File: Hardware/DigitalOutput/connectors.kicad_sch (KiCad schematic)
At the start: 3 parts, among them J1 DIGITAL OUTPUT, J3 NUCLEO LEFT, J4 NUCLEO RIGHT

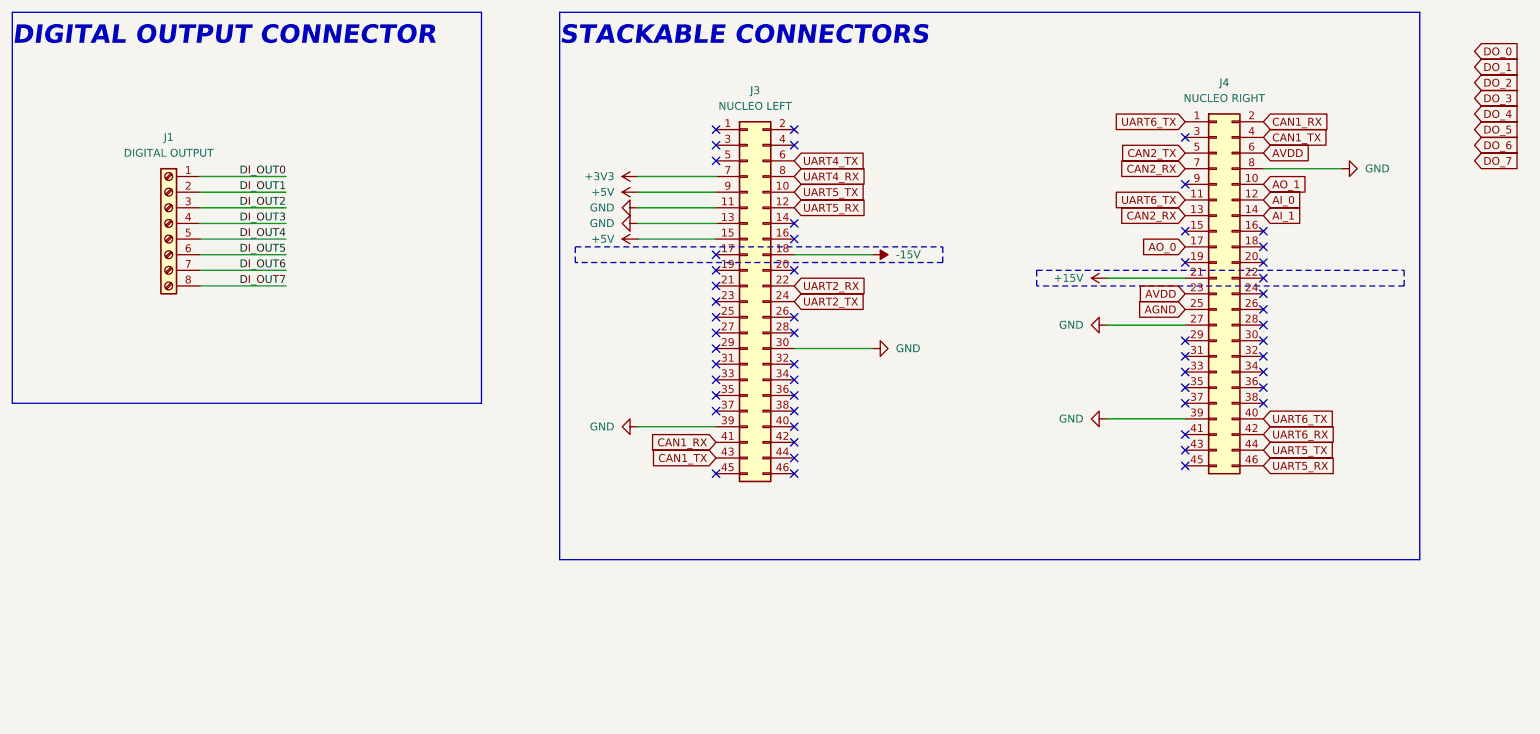
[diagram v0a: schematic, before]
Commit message: digital output & power finished
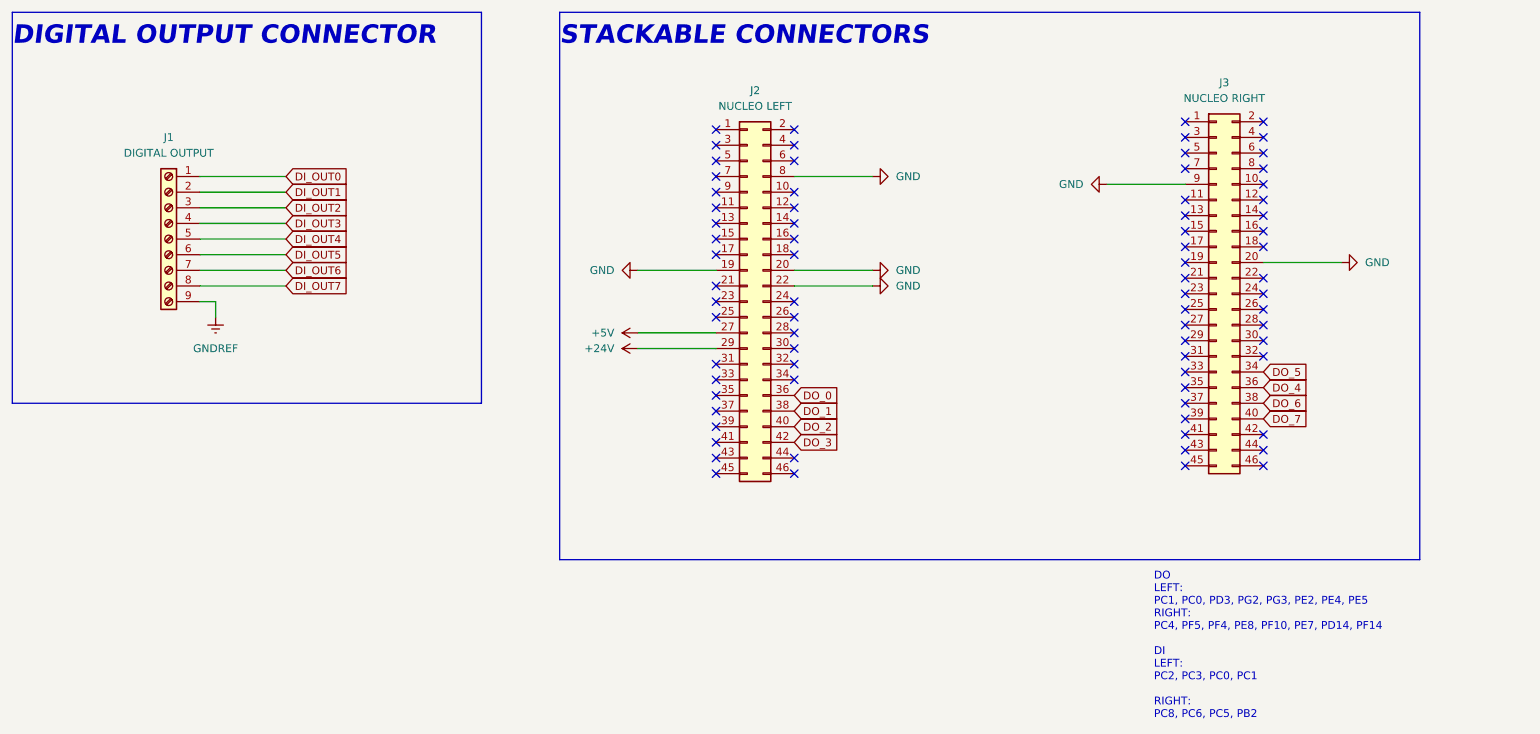
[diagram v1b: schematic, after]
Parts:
- removed J1: DIGITAL OUTPUT, PLC_STM:1725711, symbol Connector:Screw_Terminal_01x08
- added J1: DIGITAL OUTPUT, PLC_STM:1725724, symbol Connector:Screw_Terminal_01x09
- renumbered J3 to J2, J4 to J3
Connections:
- net UART2_RX is gone; now on net GND: J2.22 (Pin_22)
- net UART4_RX is gone; now on net GND: J2.8 (Pin_8)
- net +5V: now also J2.27 (Pin_27); no longer J2.15 (Pin_15), J2.9 (Pin_9)
- net DI_OUT0: now also J1.1 (Pin_1)
- net DI_OUT1: now also J1.2 (Pin_2)
- net DI_OUT2: now also J1.3 (Pin_3)
- net DI_OUT3: now also J1.4 (Pin_4)
- net DI_OUT4: now also J1.5 (Pin_5)
- net DI_OUT5: now also J1.6 (Pin_6)
- net DI_OUT6: now also J1.7 (Pin_7)
- net DI_OUT7: now also J1.8 (Pin_8)
- net DO_0: now also J2.36 (Pin_36)
- net DO_1: now also J2.38 (Pin_38)
- net DO_2: now also J2.40 (Pin_40)
- net DO_3: now also J2.42 (Pin_42)
- net DO_4: now also J3.36 (Pin_36)
- net DO_5: now also J3.34 (Pin_34)
- net DO_6: now also J3.38 (Pin_38)
- net DO_7: now also J3.40 (Pin_40)
- net GND: now also J2.19 (Pin_19), J2.20 (Pin_20), J3.20 (Pin_20), J3.9 (Pin_9); no longer J2.11 (Pin_11), J2.13 (Pin_13), J2.30 (Pin_30), J2.39 (Pin_39), J3.27 (Pin_27), J3.39 (Pin_39), J3.8 (Pin_8)
- net +24V: now reaches J2.29 (Pin_29)
- net +15V: no longer names the net of J3.21 (Pin_21)
- net +3V3: no longer names the net of J2.7 (Pin_7)
- net -15V: no longer names the net of J2.18 (Pin_18)
- net AGND: no longer names the net of J3.25 (Pin_25)
- net AI_0: no longer names the net of J3.12 (Pin_12)
- net AI_1: no longer names the net of J3.14 (Pin_14)
- net AO_0: no longer names the net of J3.17 (Pin_17)
- net AO_1: no longer names the net of J3.10 (Pin_10)
- net AVDD: no longer names the net of J3.23 (Pin_23)
- net AVDD: no longer J3.6 (Pin_6)
- net CAN1_RX: no longer names the net of J3.2 (Pin_2)
- net CAN1_RX: no longer J2.41 (Pin_41)
- net CAN1_TX: no longer names the net of J3.4 (Pin_4)
- net CAN1_TX: no longer J2.43 (Pin_43)
- net CAN2_RX: no longer names the net of J3.13 (Pin_13)
- net CAN2_RX: no longer J3.7 (Pin_7)
- net CAN2_TX: no longer names the net of J3.5 (Pin_5)
- net UART2_TX: no longer names the net of J2.24 (Pin_24)
- net UART4_TX: no longer names the net of J2.6 (Pin_6)
- net UART5_RX: no longer names the net of J3.46 (Pin_46)
- net UART5_RX: no longer J2.12 (Pin_12)
- net UART5_TX: no longer names the net of J3.44 (Pin_44)
- net UART5_TX: no longer J2.10 (Pin_10)
- net UART6_RX: no longer names the net of J3.42 (Pin_42)
- removed net UART6_TX: J3.1 (Pin_1), J3.11 (Pin_11), J3.40 (Pin_40)
- new net GNDREF: J1.9 (Pin_9)
- no-connect marks 54 -> 76
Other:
- note added: "DO LEFT: PC1, PC0, PD3, PG2, PG3, PE2, PE4, PE5 RIGHT: PC4, PF5, PF4, PE8, PF10, PE7, PD14, PF14 DI LEFT: PC2, PC3, PC0, PC1 RIGHT: PC8, PC6, PC5, PB2"

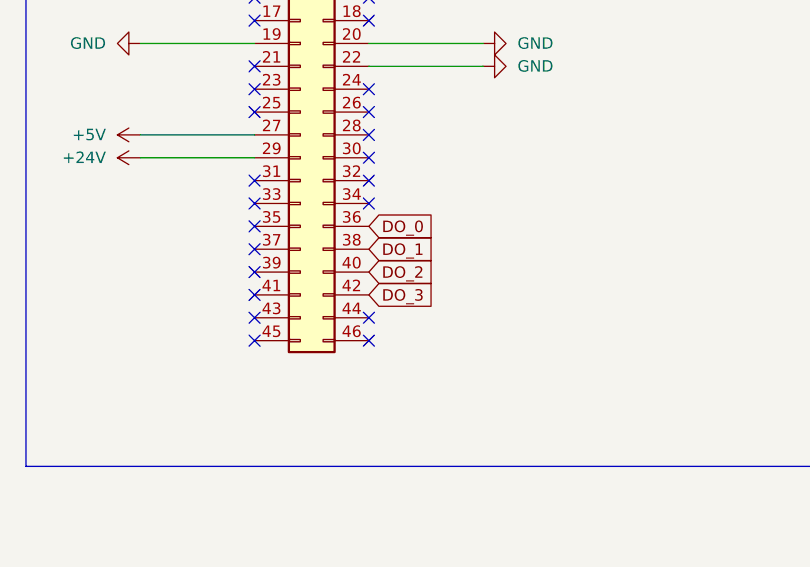
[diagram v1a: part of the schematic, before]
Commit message: small adjustments and final revision
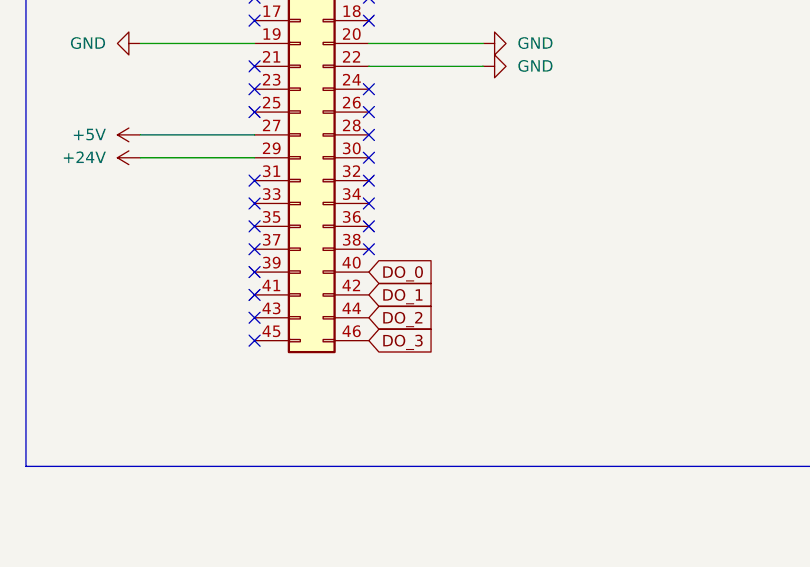
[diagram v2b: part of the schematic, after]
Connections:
- net DO_0: now also J2.40 (Pin_40); no longer J2.36 (Pin_36)
- net DO_1: now also J2.42 (Pin_42); no longer J2.38 (Pin_38)
- net DO_2: now also J2.44 (Pin_44); no longer J2.40 (Pin_40)
- net DO_3: now also J2.46 (Pin_46); no longer J2.42 (Pin_42)
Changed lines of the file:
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@@
-	)
-	(no_connect
-		(at 165.1 110.49)
 	)
 	(no_connect
@@
 	)
 	(no_connect
-		(at 165.1 113.03)
+		(at 165.1 102.87)
 	)
 	(no_connect
@@
 	)
 	(no_connect
+		(at 165.1 100.33)
+	)
+	(no_connect
 		(at 241.3 91.44)
 	)
@@
 		)
 	)
+	(global_label "DO_1"
+		(shape input)
+		(at 165.1 107.95 0)
+		(fields_autoplaced yes)
+		(effects
+			(font
+				(size 1.27 1.27)
+			)
+			(justify left)
+		)
+		(property "Intersheetrefs" "${INTERSHEET_REFS}"
+			(at 172.8628 107.95 0)
+			(effects
+				(font
+					(size 1.27 1.27)
+				)
+				(justify left)
+				(hide yes)
+			)
+		)
+	)
 	(global_label "DI_OUT1"
 		(shape input)
@@
 		)
 	)
+	(global_label "DO_5"
+		(shape input)
+		(at 241.3 96.52 0)
+		(fields_autoplaced yes)
+		(effects
+			(font
+				(size 1.27 1.27)
+			)
+			(justify left)
+		)
+		(property "Intersheetrefs" "${INTERSHEET_REFS}"
+			(at 249.0628 96.52 0)
+			(effects
+				(font
+					(size 1.27 1.27)
+				)
+				(justify left)
+				(hide yes)
+			)
+		)
+	)
 	(global_label "DO_2"
 		(shape input)
+		(at 165.1 110.49 0)
+		(fields_autoplaced yes)
+		(effects
+			(font
+				(size 1.27 1.27)
+			)
+			(justify left)
+		)
+		(property "Intersheetrefs" "${INTERSHEET_REFS}"
+			(at 172.8628 110.49 0)
+			(effects
+				(font
+					(size 1.27 1.27)
+				)
+				(justify left)
+				(hide yes)
+			)
+		)
+	)
+	(global_label "DI_OUT2"
+		(shape input)
+		(at 82.55 69.85 0)
+		(fields_autoplaced yes)
+		(effects
+			(font
+				(size 1.27 1.27)
+			)
+			(justify left)
+		)
+		(property "Intersheetrefs" "${INTERSHEET_REFS}"
+			(at 93.2157 69.85 0)
+			(effects
+				(font
+					(size 1.27 1.27)
+				)
+				(justify left)
+				(hide yes)
+			)
+		)
+	)
+	(global_label "DO_4"
+		(shape input)
+		(at 241.3 99.06 0)
+		(fields_autoplaced yes)
+		(effects
+			(font
+				(size 1.27 1.27)
+			)
+			(justify left)
+		)
+		(property "Intersheetrefs" "${INTERSHEET_REFS}"
+			(at 249.0628 99.06 0)
+			(effects
+				(font
+					(size 1.27 1.27)
+				)
+				(justify left)
+				(hide yes)
+			)
+		)
+	)
+	(global_label "DI_OUT3"
+		(shape input)
+		(at 82.55 72.39 0)
+		(fields_autoplaced yes)
+		(effects
+			(font
+				(size 1.27 1.27)
+			)
+			(justify left)
+		)
+		(property "Intersheetrefs" "${INTERSHEET_REFS}"
+			(at 93.2157 72.39 0)
+			(effects
+				(font
+					(size 1.27 1.27)
+				)
+				(justify left)
+				(hide yes)
+			)
+		)
+	)
+	(global_label "DO_7"
+		(shape input)
+		(at 241.3 104.14 0)
+		(fields_autoplaced yes)
+		(effects
+			(font
+				(size 1.27 1.27)
+			)
+			(justify left)
+		)
+		(property "Intersheetrefs" "${INTERSHEET_REFS}"
+			(at 249.0628 104.14 0)
+			(effects
+				(font
+					(size 1.27 1.27)
+				)
+				(justify left)
+				(hide yes)
+			)
+		)
+	)
+	(global_label "DO_0"
+		(shape input)
 		(at 165.1 105.41 0)
 		(fields_autoplaced yes)
@@
 		)
 	)
-	(global_label "DO_5"
-		(shape input)
-		(at 241.3 96.52 0)
-		(fields_autoplaced yes)
-		(effects
-			(font
-				(size 1.27 1.27)
-			)
-			(justify left)
-		)
-		(property "Intersheetrefs" "${INTERSHEET_REFS}"
-			(at 249.0628 96.52 0)
-			(effects
-				(font
-					(size 1.27 1.27)
-				)
-				(justify left)
-				(hide yes)
-			)
-		)
-	)
-	(global_label "DI_OUT2"
-		(shape input)
-		(at 82.55 69.85 0)
-		(fields_autoplaced yes)
-		(effects
-			(font
-				(size 1.27 1.27)
-			)
-			(justify left)
-		)
-		(property "Intersheetrefs" "${INTERSHEET_REFS}"
-			(at 93.2157 69.85 0)
-			(effects
-				(font
-					(size 1.27 1.27)
-				)
-				(justify left)
-				(hide yes)
-			)
-		)
-	)
-	(global_label "DO_0"
-		(shape input)
-		(at 165.1 100.33 0)
-		(fields_autoplaced yes)
-		(effects
-			(font
-				(size 1.27 1.27)
-			)
-			(justify left)
-		)
-		(property "Intersheetrefs" "${INTERSHEET_REFS}"
-			(at 172.8628 100.33 0)
-			(effects
-				(font
-					(size 1.27 1.27)
-				)
-				(justify left)
-				(hide yes)
-			)
-		)
-	)
-	(global_label "DO_4"
-		(shape input)
-		(at 241.3 99.06 0)
-		(fields_autoplaced yes)
-		(effects
-			(font
-				(size 1.27 1.27)
-			)
-			(justify left)
-		)
-		(property "Intersheetrefs" "${INTERSHEET_REFS}"
-			(at 249.0628 99.06 0)
-			(effects
-				(font
-					(size 1.27 1.27)
-				)
-				(justify left)
-				(hide yes)
-			)
-		)
-	)
-	(global_label "DI_OUT3"
-		(shape input)
-		(at 82.55 72.39 0)
-		(fields_autoplaced yes)
-		(effects
-			(font
-				(size 1.27 1.27)
-			)
-			(justify left)
-		)
-		(property "Intersheetrefs" "${INTERSHEET_REFS}"
-			(at 93.2157 72.39 0)
-			(effects
-				(font
-					(size 1.27 1.27)
-				)
-				(justify left)
-				(hide yes)
-			)
-		)
-	)
-	(global_label "DO_7"
-		(shape input)
-		(at 241.3 104.14 0)
-		(fields_autoplaced yes)
-		(effects
-			(font
-				(size 1.27 1.27)
-			)
-			(justify left)
-		)
-		(property "Intersheetrefs" "${INTERSHEET_REFS}"
-			(at 249.0628 104.14 0)
-			(effects
-				(font
-					(size 1.27 1.27)
-				)
-				(justify left)
-				(hide yes)
-			)
-		)
-	)
 	(global_label "DI_OUT0"
 		(shape input)
@@
 	(global_label "DO_3"
 		(shape input)
-		(at 165.1 107.95 0)
-		(fields_autoplaced yes)
-		(effects
-			(font
-				(size 1.27 1.27)
-			)
-			(justify left)
-		)
-		(property "Intersheetrefs" "${INTERSHEET_REFS}"
-			(at 172.8628 107.95 0)
+		(at 165.1 113.03 0)
+		(fields_autoplaced yes)
+		(effects
+			(font
+				(size 1.27 1.27)
+			)
+			(justify left)
+		)
+		(property "Intersheetrefs" "${INTERSHEET_REFS}"
+			(at 172.8628 113.03 0)
 			(effects
 				(font
@@
 			(effects
 				(font
-					(size 1.27 1.27)
-				)
-				(justify left)
-				(hide yes)
-			)
-		)
-	)
-	(global_label "DO_1"
-		(shape input)
-		(at 165.1 102.87 0)
-		(fields_autoplaced yes)
-		(effects
-			(font
-				(size 1.27 1.27)
-			)
-			(justify left)
-		)
-		(property "Intersheetrefs" "${INTERSHEET_REFS}"
-			(at 172.8628 102.87 0)
-			(effects
-				(font
